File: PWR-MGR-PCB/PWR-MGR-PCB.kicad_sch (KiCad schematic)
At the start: 23 parts, among them J1 USB_C_Receptacle_USB2.0_16P, J2 Battery_1x2, J3 Conn_01x01_Pin, J4 Conn_01x01_Pin, J5 Conn_01x01_Pin, J6 Conn_01x01_Pin, U1 USBLC6-2SC6, U2 TLV75533PDBV, U3 BQ24074RGT

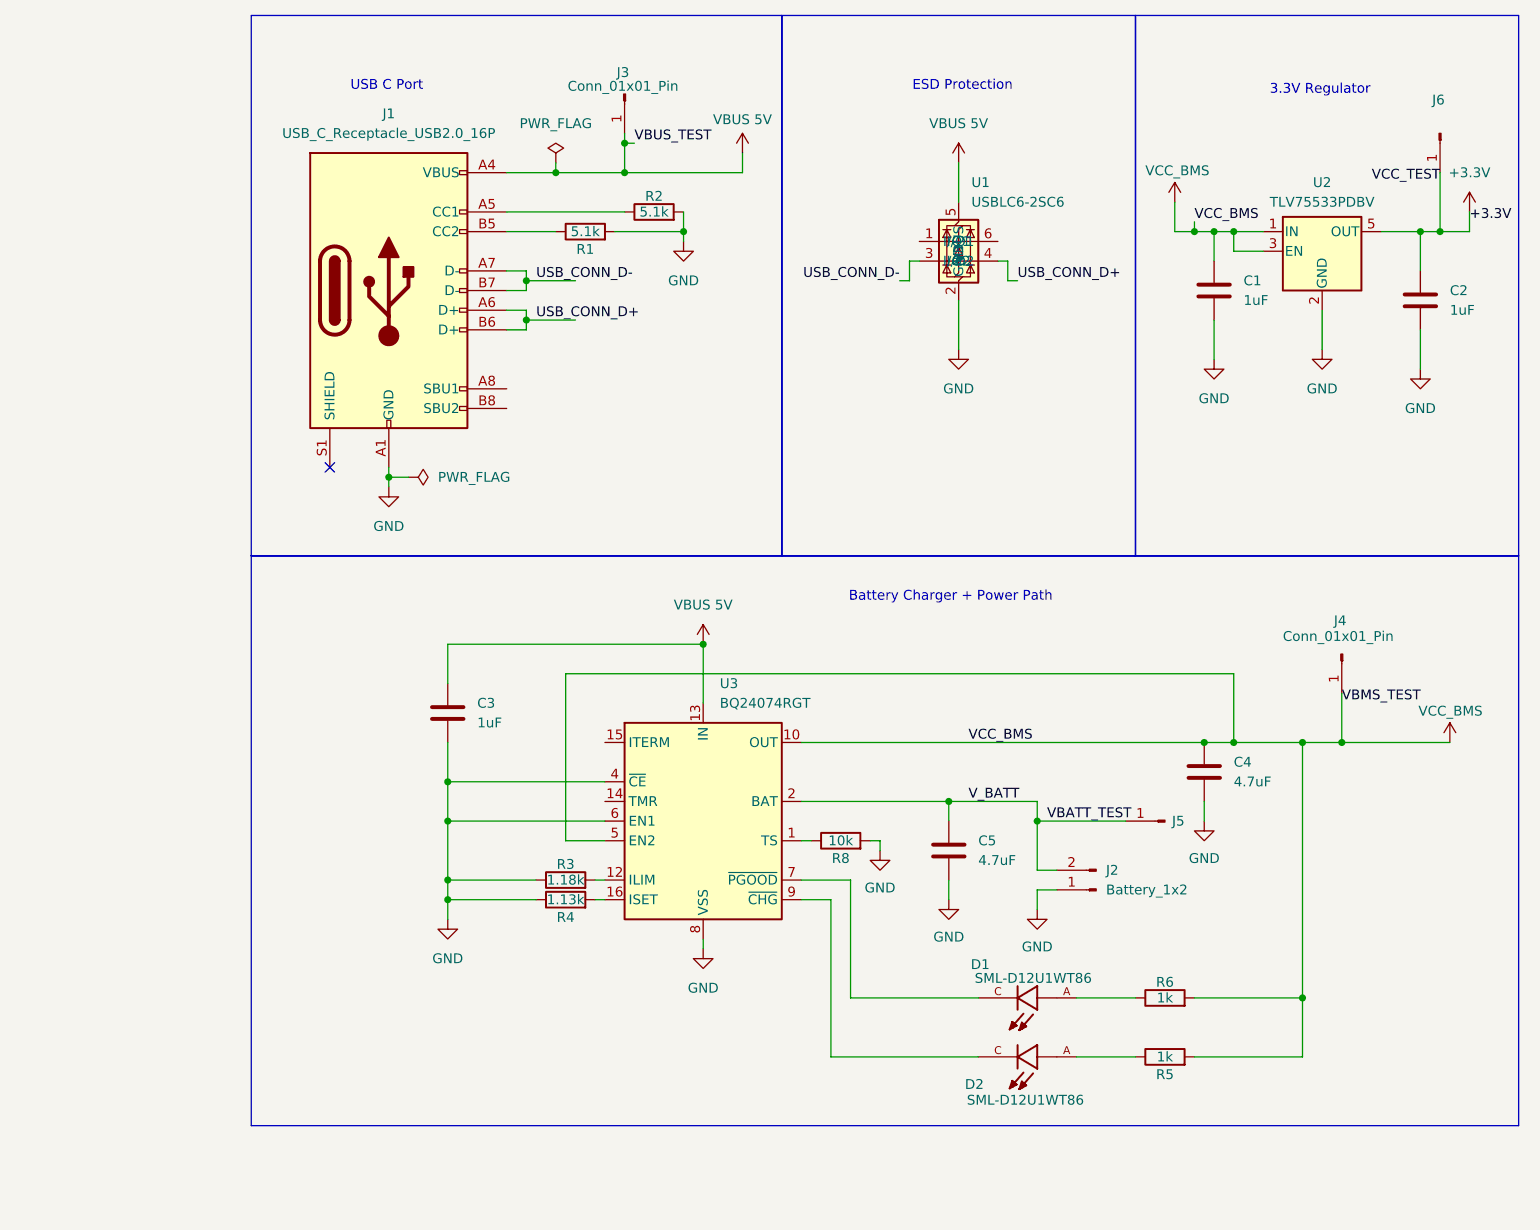
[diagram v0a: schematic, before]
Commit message: Sync latest fixes
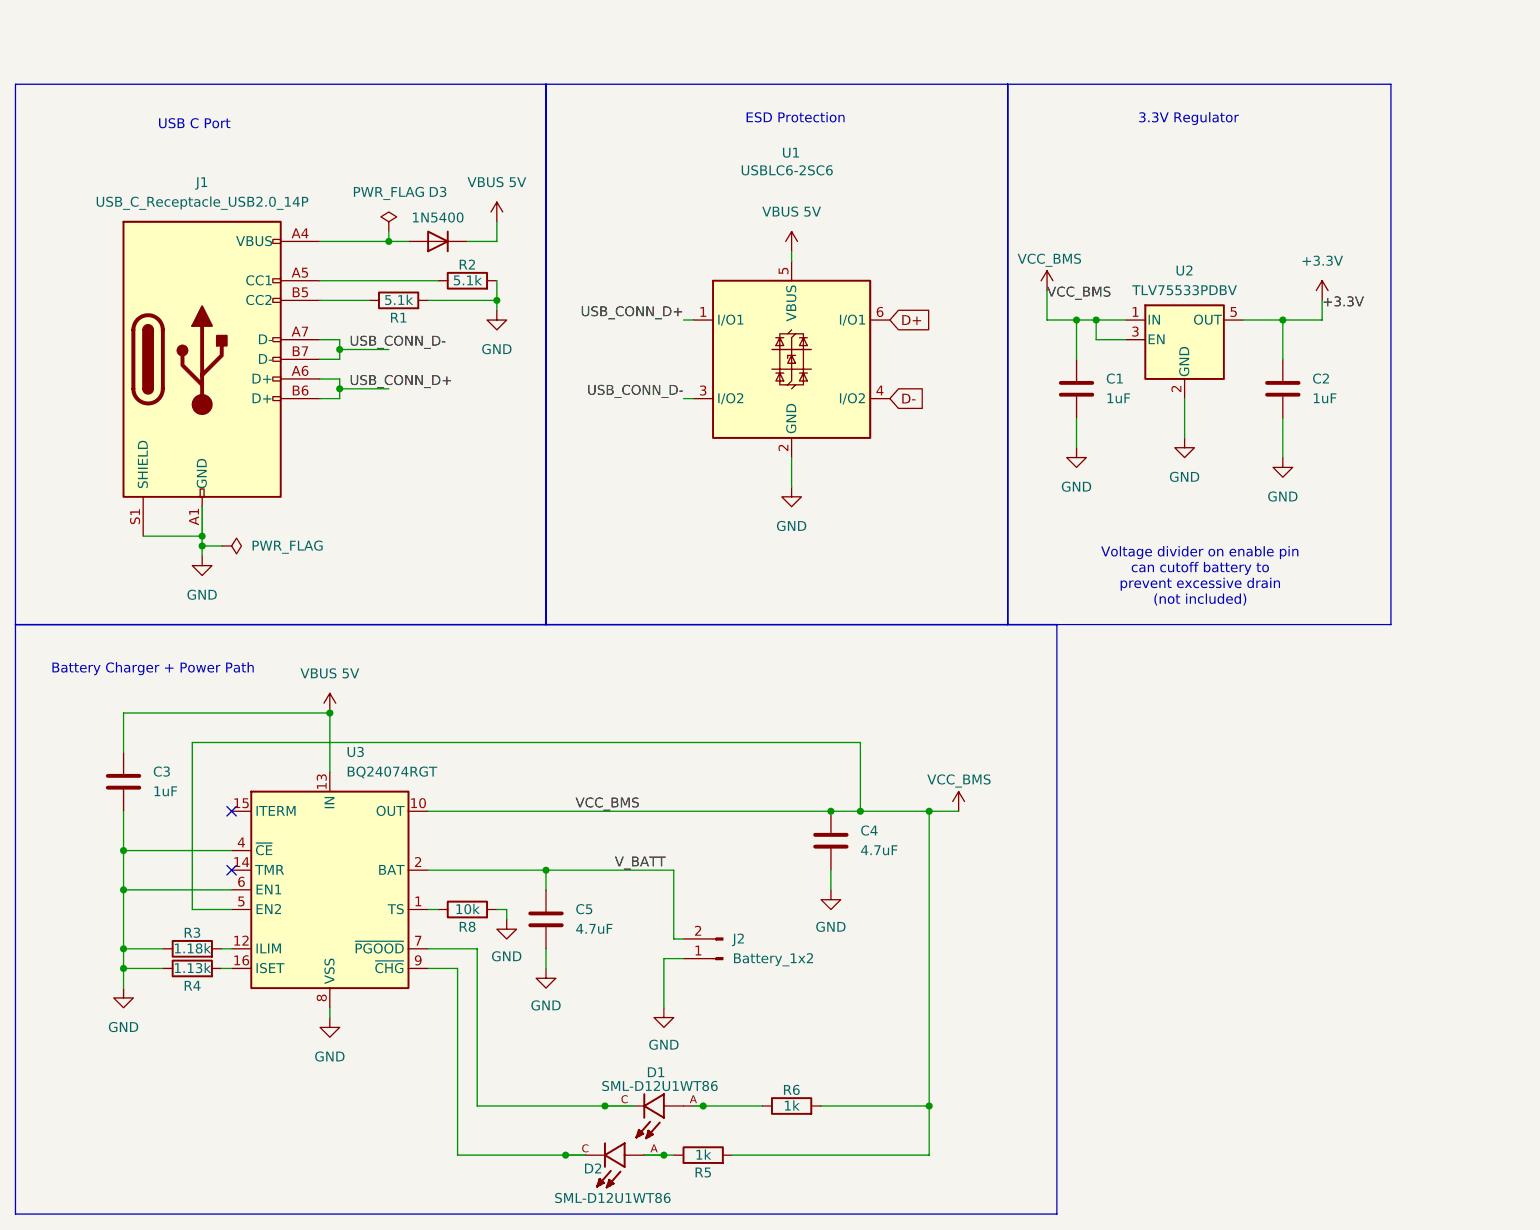
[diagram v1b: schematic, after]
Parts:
- removed J1: USB_C_Receptacle_USB2.0_16P, Connector_USB:USB_C_Receptacle_GCT_USB4105-xx-A_16P_TopMnt_Horizontal, symbol Connector:USB_C_Receptacle_USB2.0_16P
- removed J3, J4, J5, J6: Conn_01x01_Pin, Connector_PinSocket_2.54mm:PinSocket_1x01_P2.54mm_Vertical, symbol Connector:Conn_01x01_Pin
- added D3: 1N5400, Diode_THT:D_DO-201AD_P15.24mm_Horizontal, symbol Diode:1N5400
- added J1: USB_C_Receptacle_USB2.0_14P, Connector_USB:USB_C_Receptacle_GCT_USB4105-xx-A_16P_TopMnt_Horizontal, symbol Connector:USB_C_Receptacle_USB2.0_14P
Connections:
- net GND: now also J1.A1 (GND), J1.A12 (GND), J1.B1 (GND), J1.B12 (GND), J1.S1 (SHIELD)
- net USB_CONN_D+: now also U1.1 (I/O1), J1.A6 (D+), J1.B6 (D+); no longer U1.4 (I/O2)
- net USB_CONN_D-: now also J1.A7 (D-), J1.B7 (D-)
- net VBUS 5V: now also D3.1 (K)
- net at R2.1: now also J1.A5 (CC1)
- net at R1.1: now also J1.B5 (CC2)
- net D+: now reaches U1.6 (I/O1)
- net VBATT_TEST renamed V_BATT
- new net: D3.2 (A), J1.A4 (VBUS), J1.A9 (VBUS), J1.B4 (VBUS), J1.B9 (VBUS)
- new net D-: U1.4 (I/O2)
- no-connect marks 1 -> 2
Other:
- note added: "Voltage divider on enable pin can cutoff battery to prevent excessive drain (not included)"
- moved on the sheet: C1, C2, C3, C4, C5, D1, D2, J2, R1, R2, R3, R4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
